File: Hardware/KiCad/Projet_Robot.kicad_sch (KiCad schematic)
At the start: 0 parts

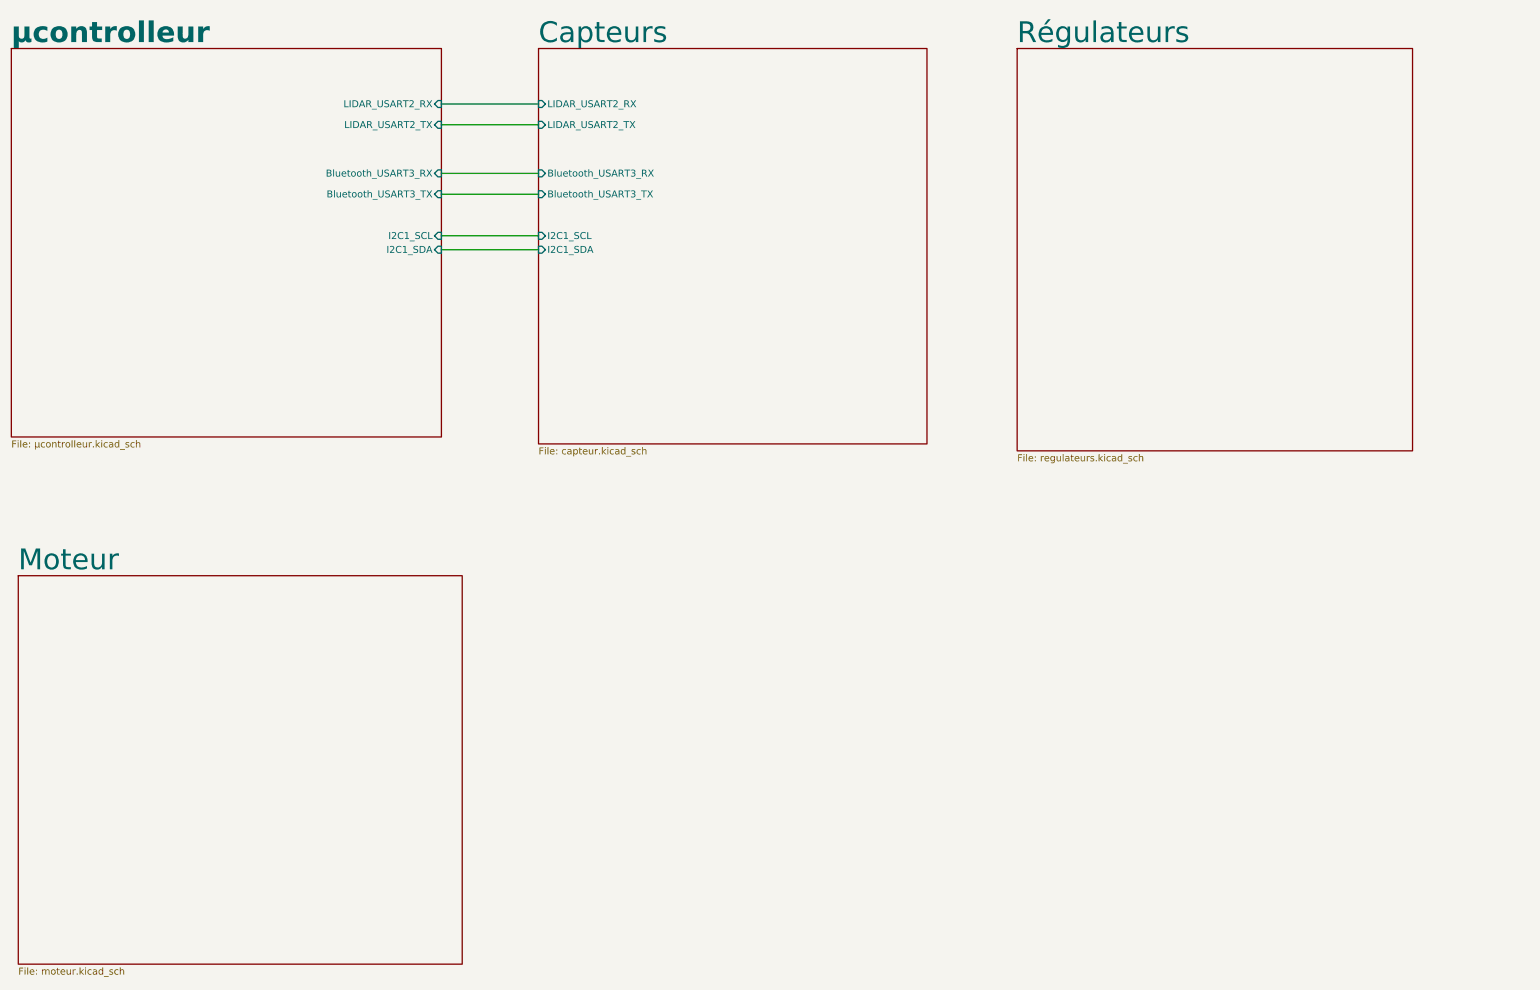
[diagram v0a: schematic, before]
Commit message: change
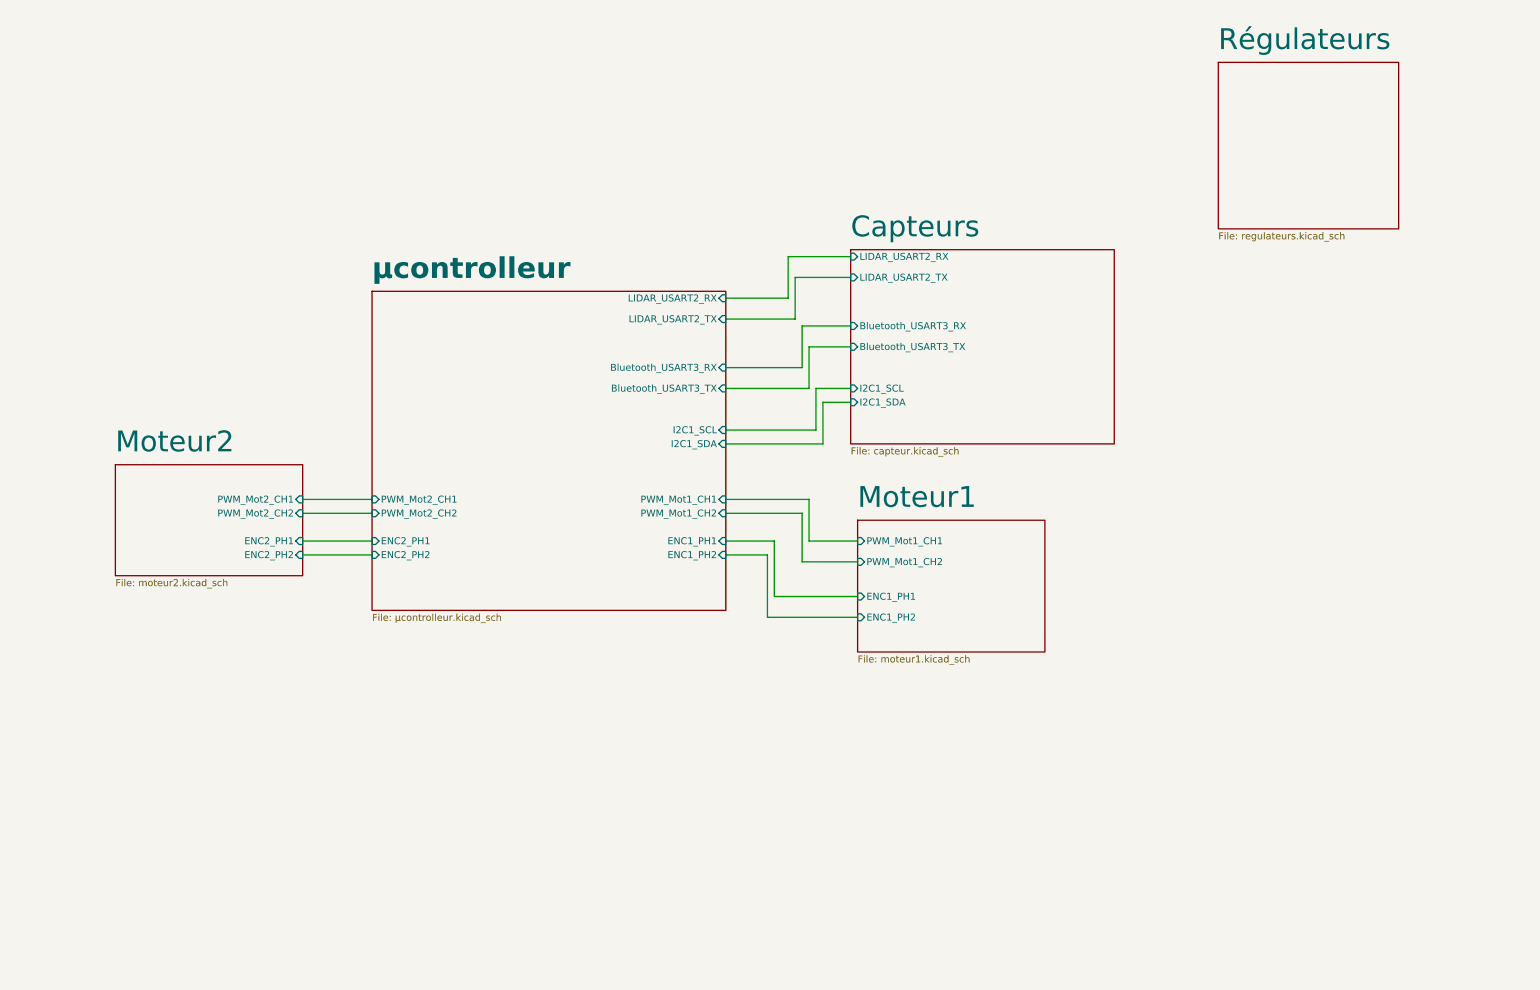
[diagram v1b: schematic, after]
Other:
- removed sheet Moteur
- added sheet Moteur1 (moteur1.kicad_sch)
- added sheet Moteur2 (moteur2.kicad_sch)
- sheet µcontrolleur ports: added ENC1_PH1, ENC1_PH2, ENC2_PH1, ENC2_PH2, PWM_Mot1_CH1, PWM_Mot1_CH2, PWM_Mot2_CH1, PWM_Mot2_CH2; removed none

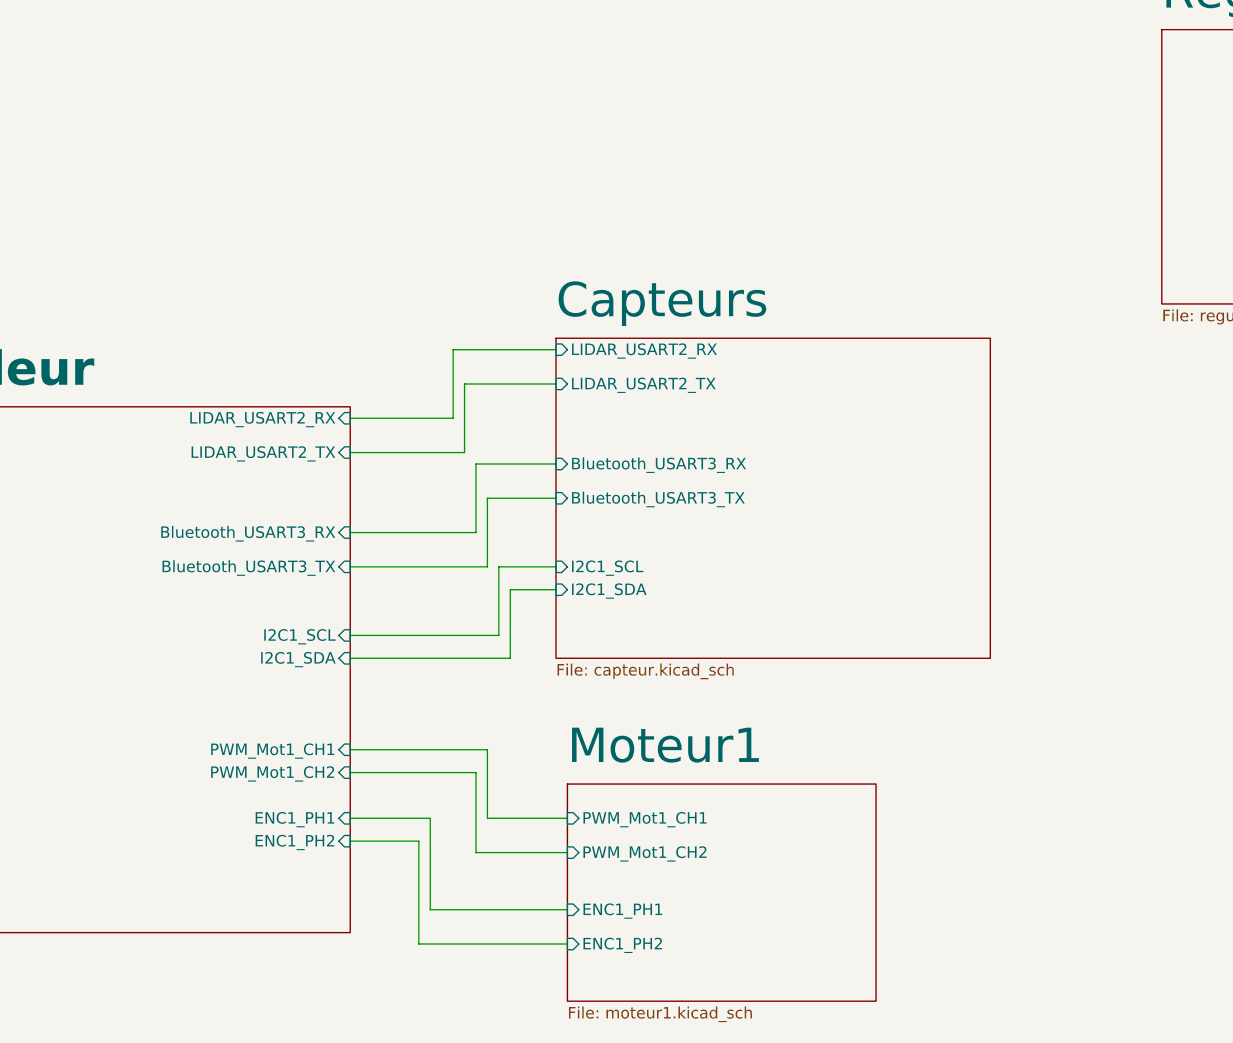
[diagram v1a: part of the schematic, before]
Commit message: Robot
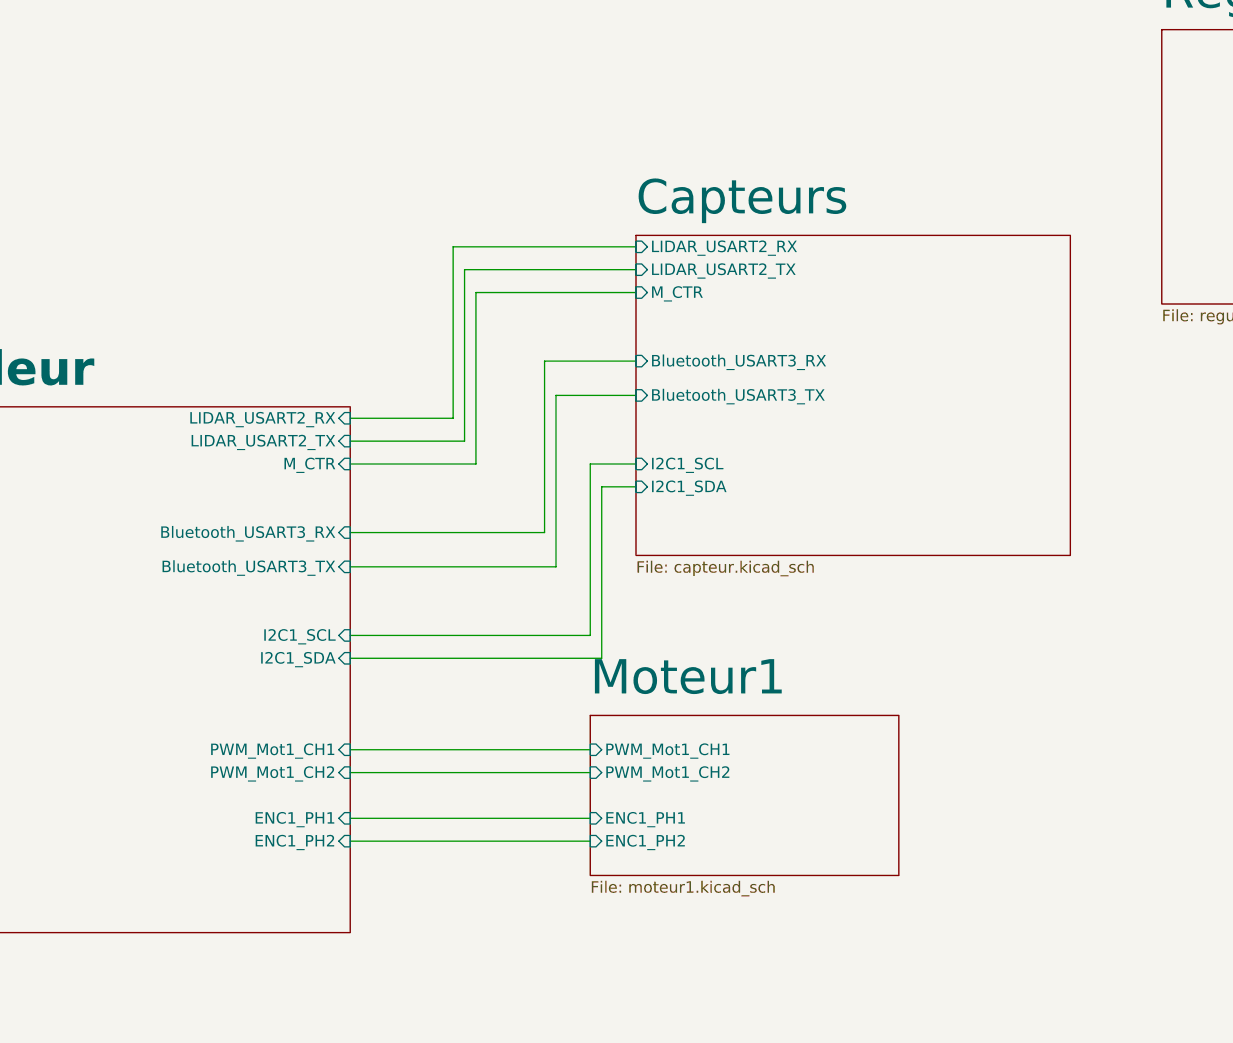
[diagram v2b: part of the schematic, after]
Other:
- sheet Capteurs ports: added M_CTR; removed none
- sheet µcontrolleur ports: added M_CTR; removed none

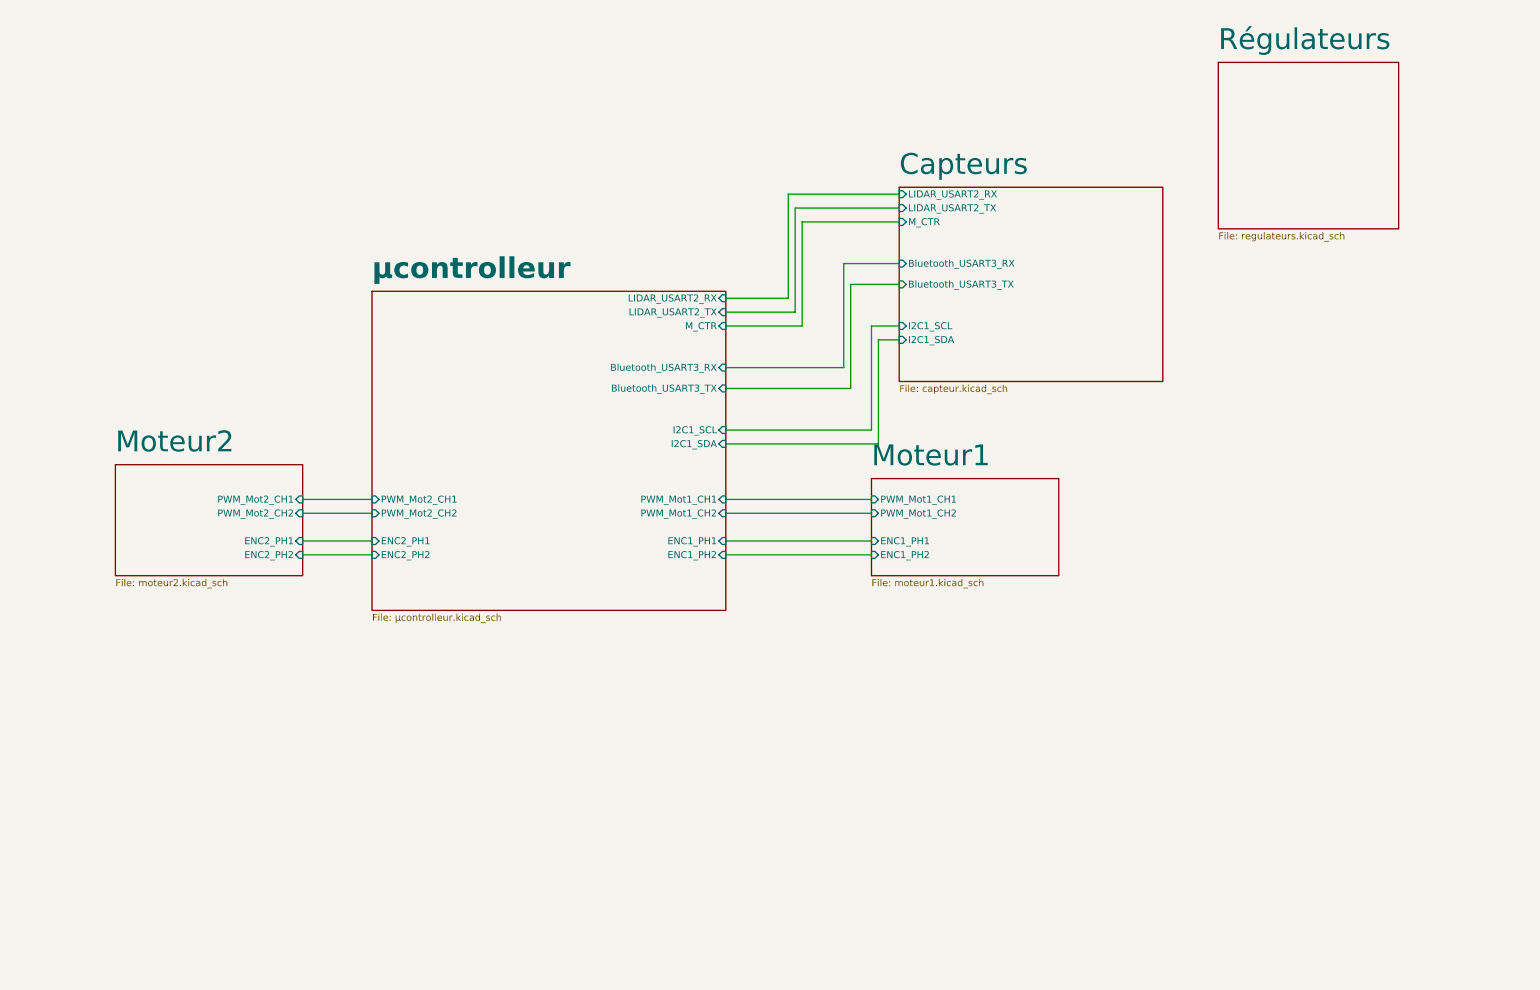
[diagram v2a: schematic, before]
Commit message: commit
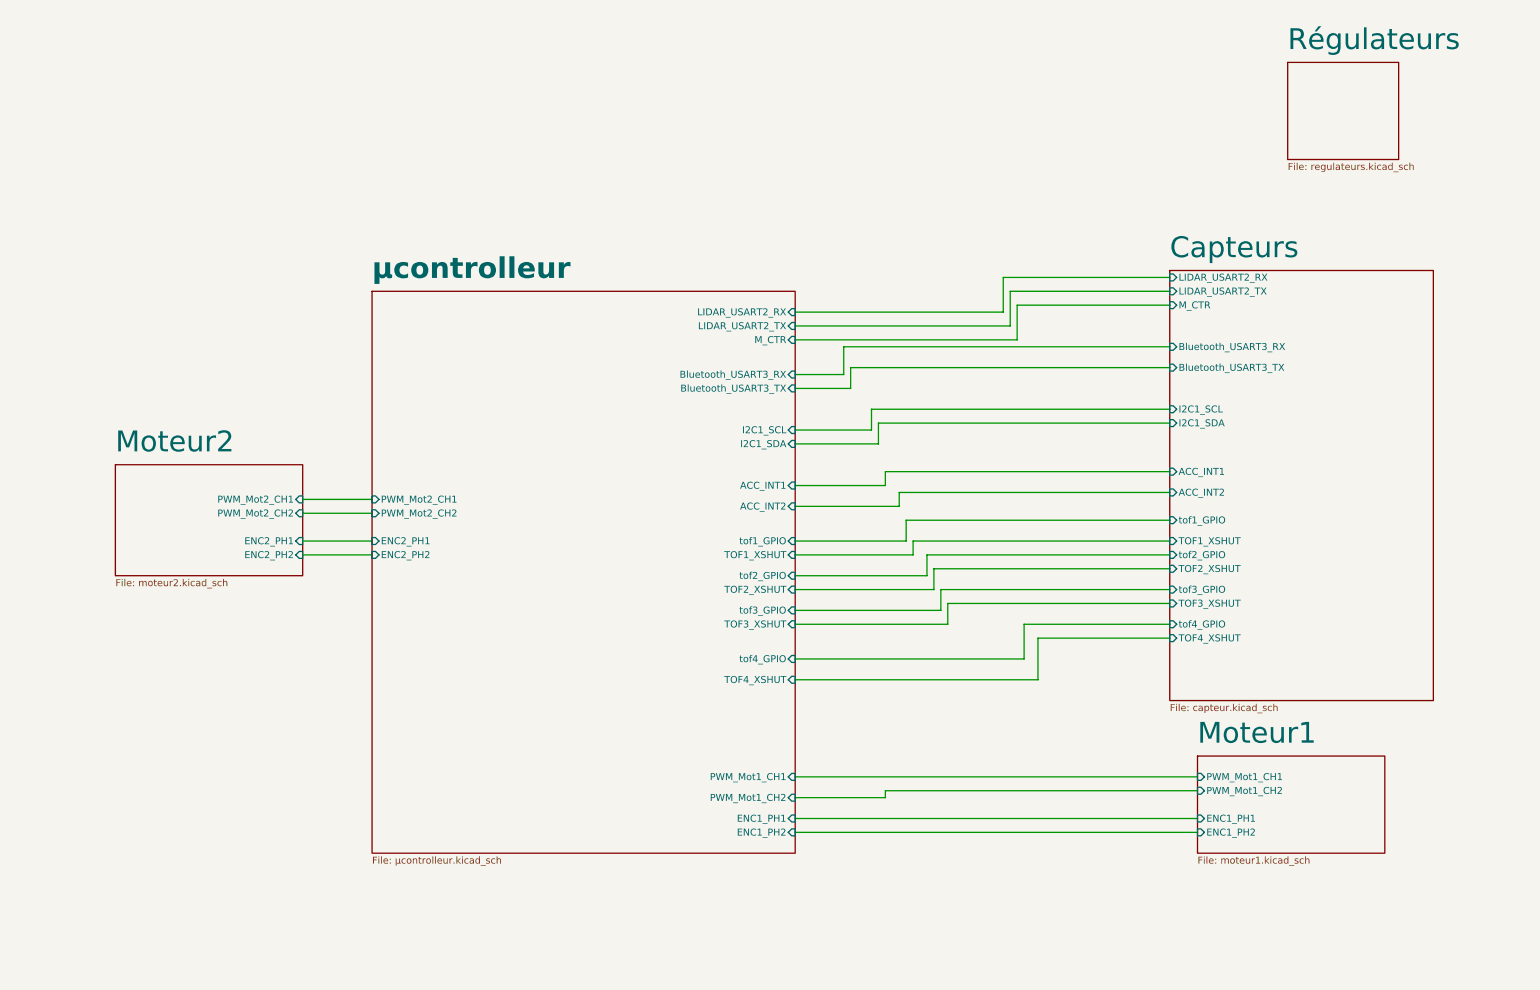
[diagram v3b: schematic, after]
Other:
- sheet Capteurs ports: added ACC_INT1, ACC_INT2, TOF1_XSHUT, TOF2_XSHUT, TOF3_XSHUT, TOF4_XSHUT, tof1_GPIO, tof2_GPIO, tof3_GPIO, tof4_GPIO; removed none
- sheet µcontrolleur ports: added ACC_INT1, ACC_INT2, TOF1_XSHUT, TOF2_XSHUT, TOF3_XSHUT, TOF4_XSHUT, tof1_GPIO, tof2_GPIO, tof3_GPIO, tof4_GPIO; removed none
